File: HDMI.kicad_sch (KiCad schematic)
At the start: 8 parts, among them IC8 TPS2557QDRBTQ1, J4 HDMI_D_1.4

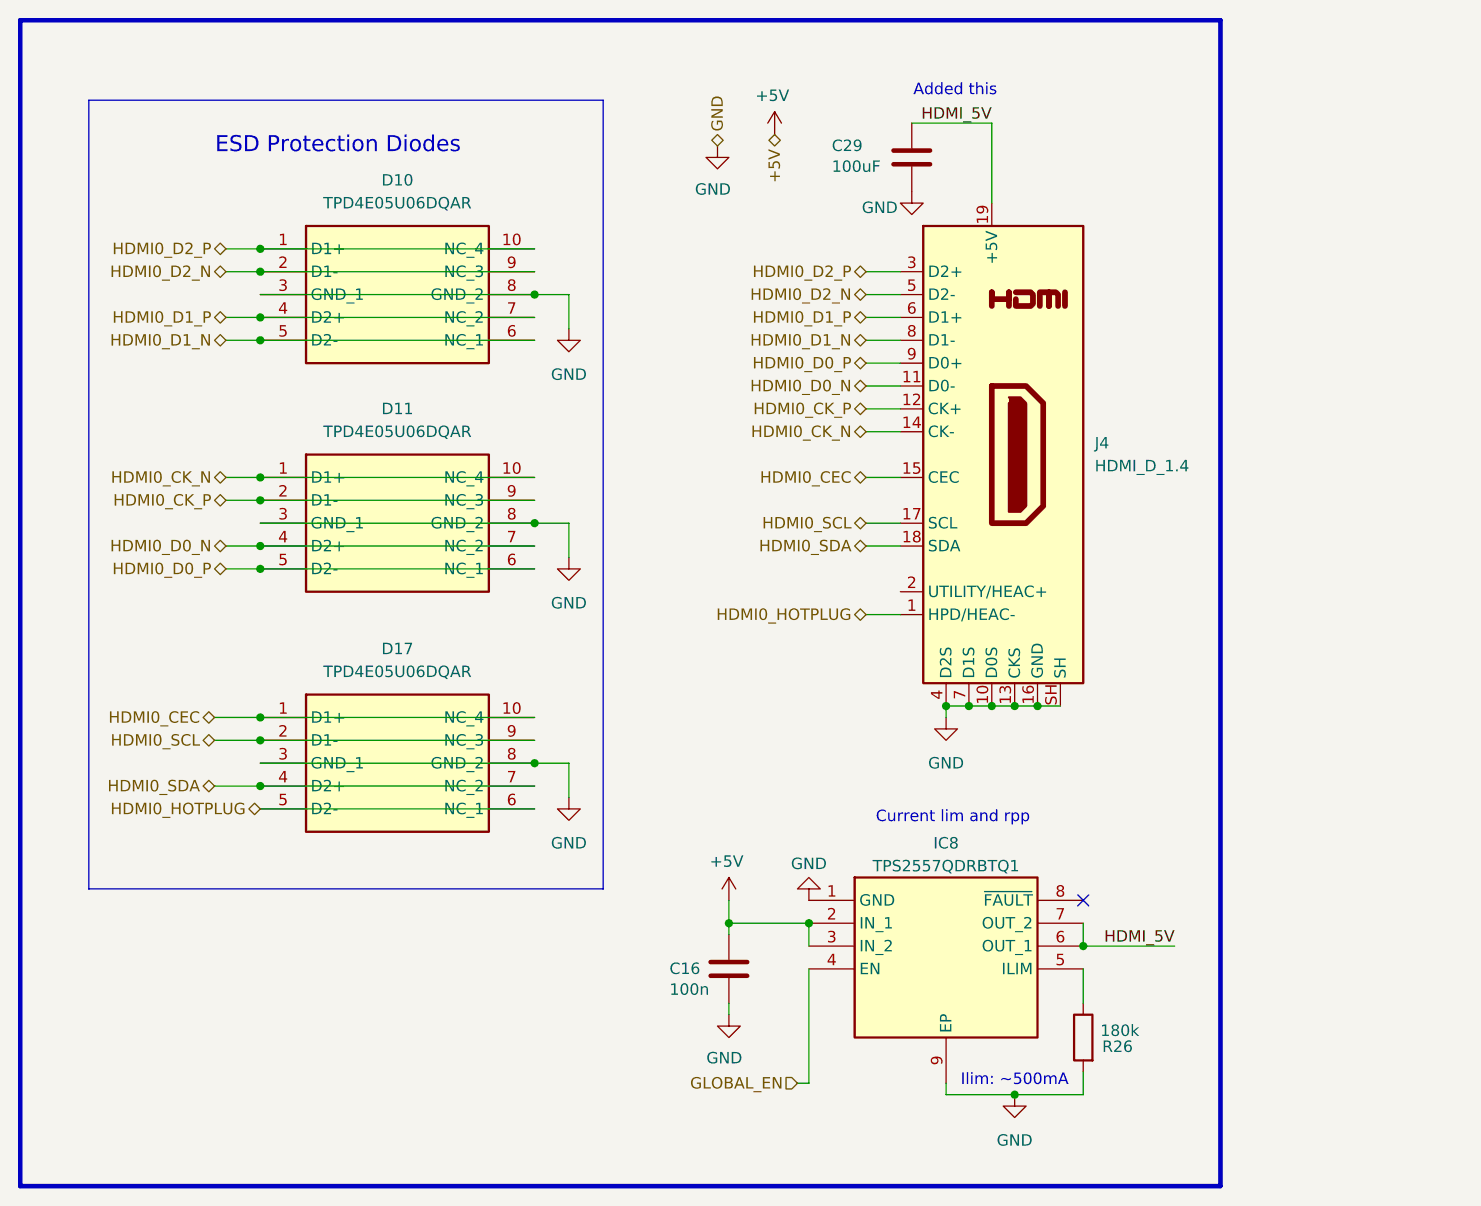
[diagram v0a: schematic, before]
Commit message: wow everything could not be worse
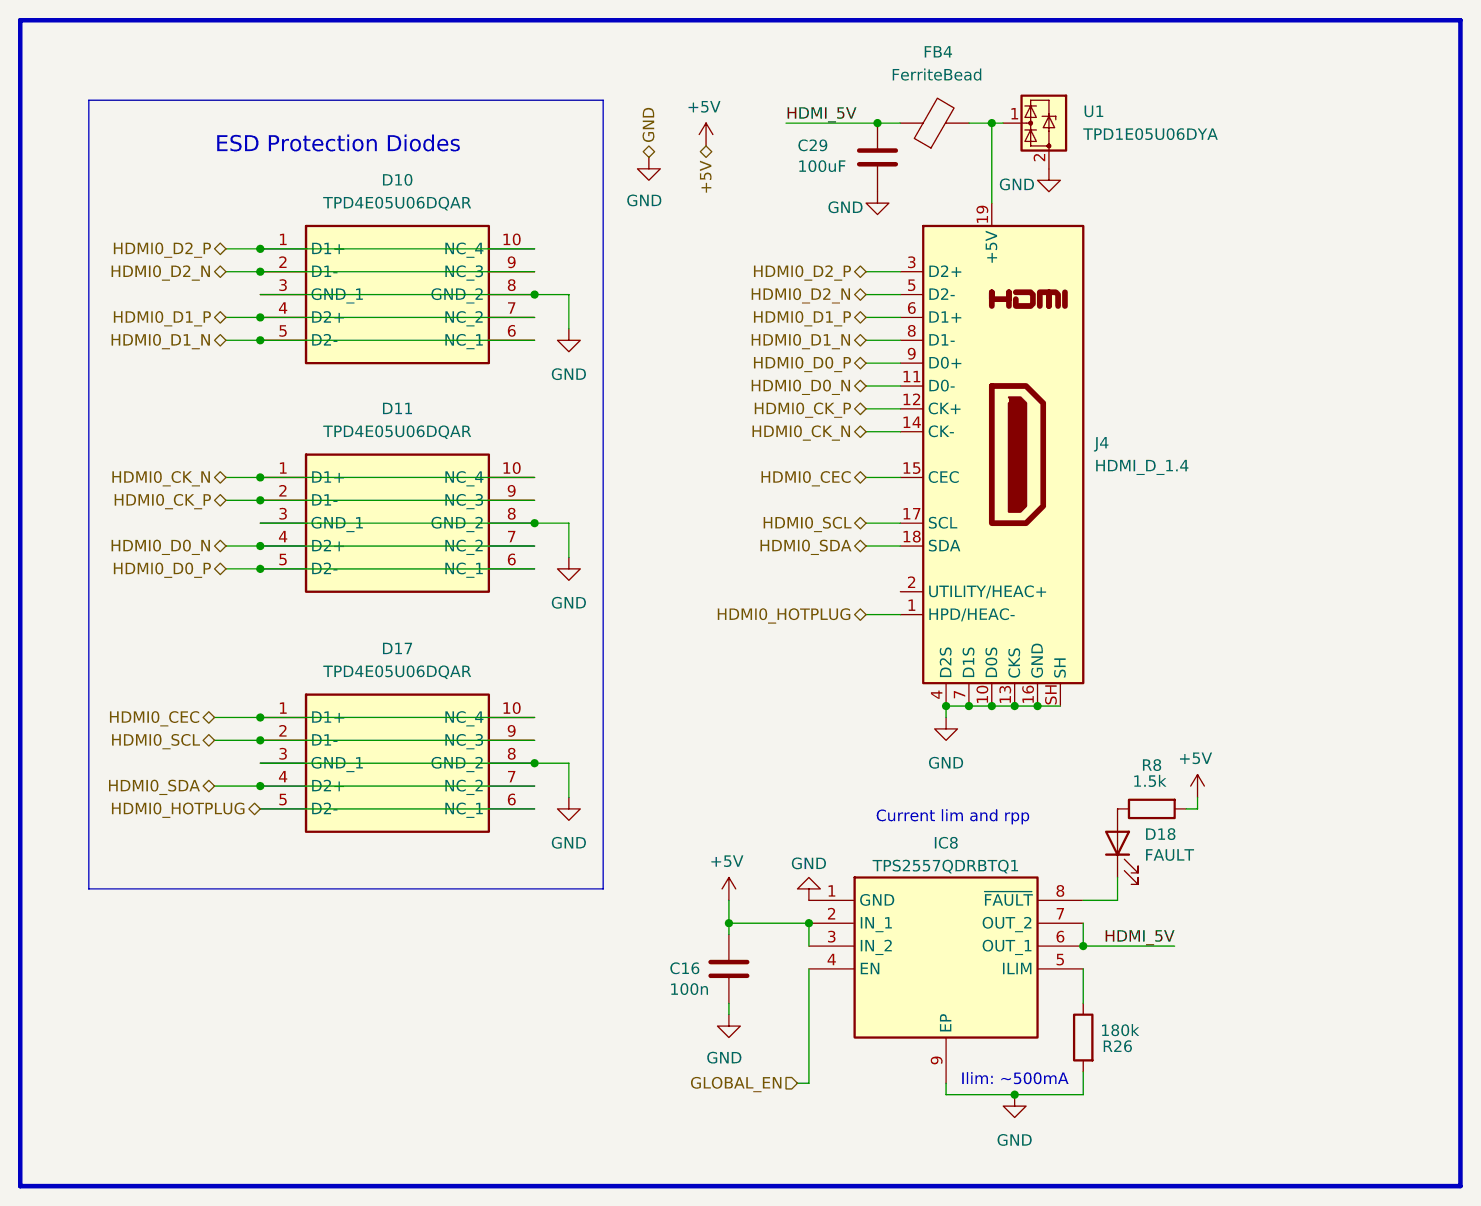
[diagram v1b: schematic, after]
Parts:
- added D18: FAULT, LED_SMD:LED_0603_1608Metric_Pad1.05x0.95mm_HandSolder, symbol Device:LED
- added FB4: FerriteBead, Inductor_SMD:L_1206_3216Metric, symbol Device:FerriteBead
- added R8: 1.5k, Resistor_SMD:R_0603_1608Metric_Pad0.98x0.95mm_HandSolder, symbol Device:R
- added U1: TPD1E05U06DYA, Diode_SMD:D_SOD-523, symbol Power_Protection:TPD1E05U06DYA
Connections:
- net +5V: now also R8.2
- net GND: now also U1.2 (GND)
- net HDMI_5V: now also FB4.1; no longer J4.19 (+5V)
- net at IC8.8 (~{FAULT}): now also D18.1 (K)
- new net: D18.2 (A), R8.1
- new net: FB4.2, J4.19 (+5V), U1.1 (I/O)
- no-connect marks 1 -> 0
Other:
- note removed: "Added this"
- moved on the sheet: C29

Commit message: my life could not be worse right now
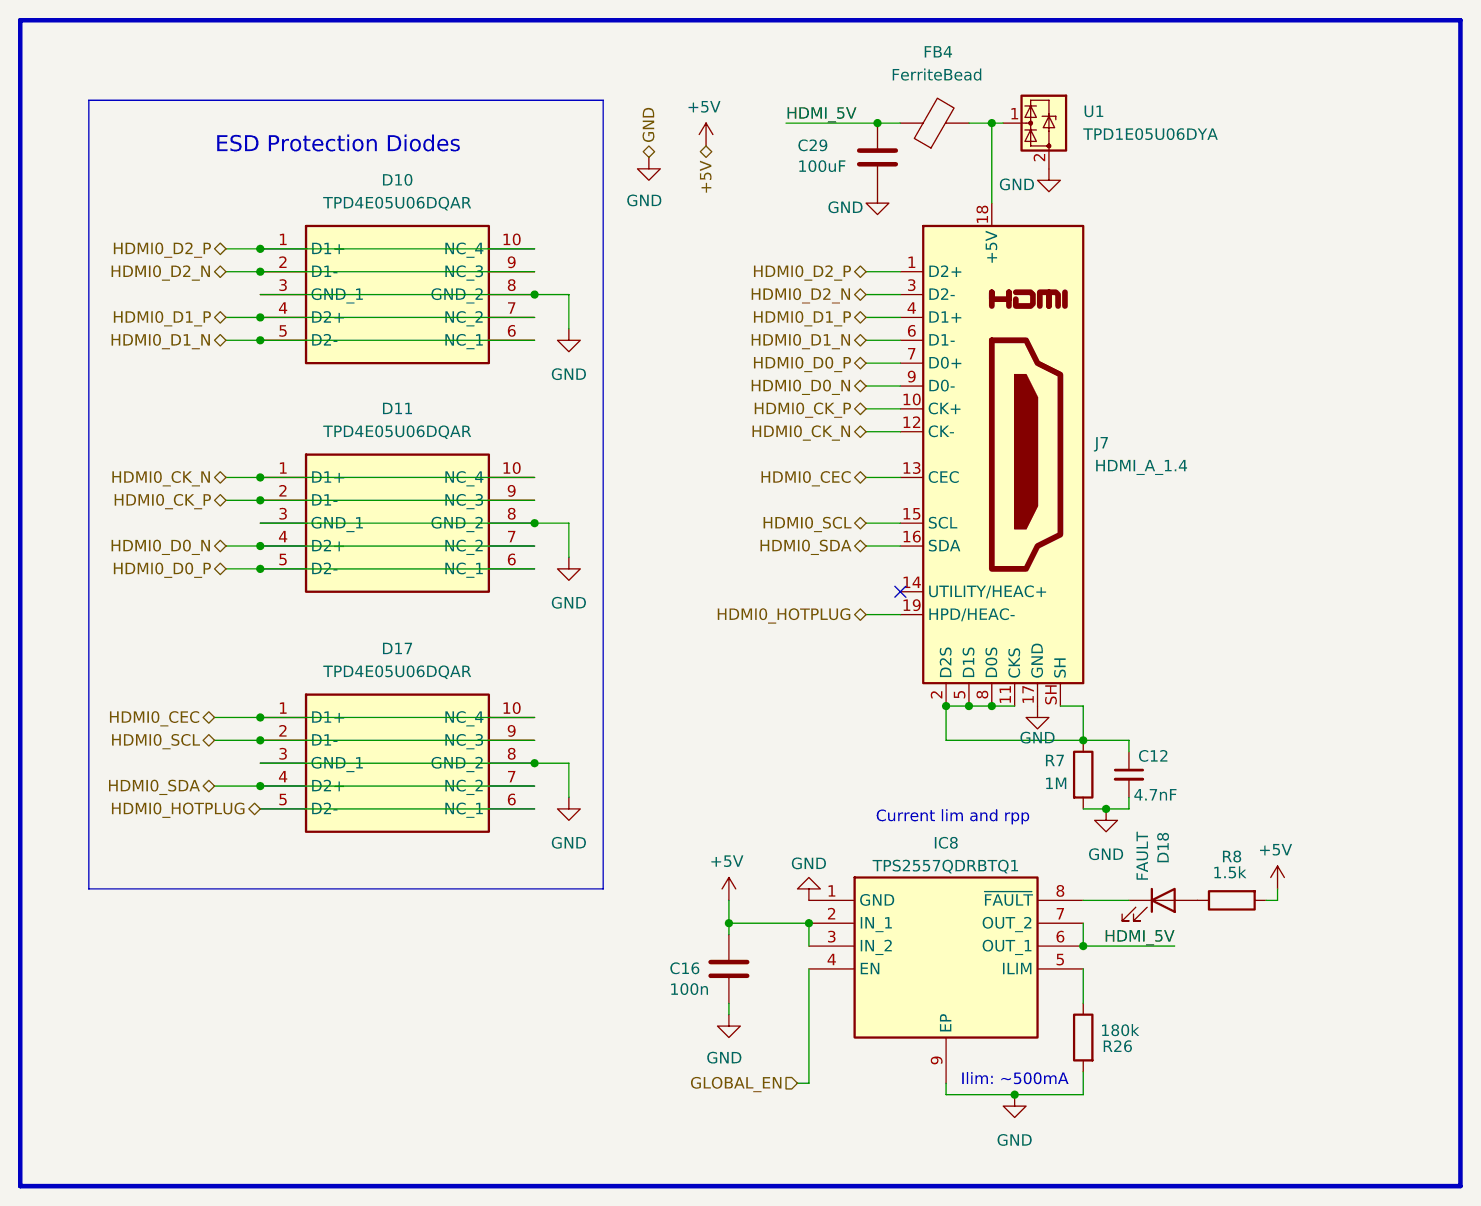
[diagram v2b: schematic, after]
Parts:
- removed J4: HDMI_D_1.4, Connector_Video:HDMI_Micro-D_Molex_46765-1x01, symbol Connector:HDMI_D_1.4
- added C12: 4.7nF, Capacitor_SMD:C_0603_1608Metric_Pad1.08x0.95mm_HandSolder, symbol Device:C_Small
- added J7: HDMI_A_1.4, Connector_Video:HDMI_A_Molex_208658-1001_Horizontal, symbol Connector:HDMI_A_1.4
- added R7: 1M, Resistor_SMD:R_0603_1608Metric_Pad0.98x0.95mm_HandSolder, symbol Device:R
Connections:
- net GND: now also C12.2, J7.17 (GND), R7.2
- net HDMI0_CEC: now also J7.13 (CEC)
- net HDMI0_CK_N: now also J7.12 (CK-)
- net HDMI0_CK_P: now also J7.10 (CK+)
- net HDMI0_D0_N: now also J7.9 (D0-)
- net HDMI0_D0_P: now also J7.7 (D0+)
- net HDMI0_D1_N: now also J7.6 (D1-)
- net HDMI0_D1_P: now also J7.4 (D1+)
- net HDMI0_D2_N: now also J7.3 (D2-)
- net HDMI0_D2_P: now also J7.1 (D2+)
- net HDMI0_HOTPLUG: now also J7.19 (HPD/HEAC-)
- net HDMI0_SCL: now also J7.15 (SCL)
- net HDMI0_SDA: now also J7.16 (SDA)
- net at FB4.2, U1.1 (I/O): now also J7.18 (+5V)
- new net: C12.1, J7.11 (CKS), J7.2 (D2S), J7.5 (D1S), J7.8 (D0S), J7.SH, R7.1
- no-connect marks 0 -> 1
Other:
- moved on the sheet: D18, R8

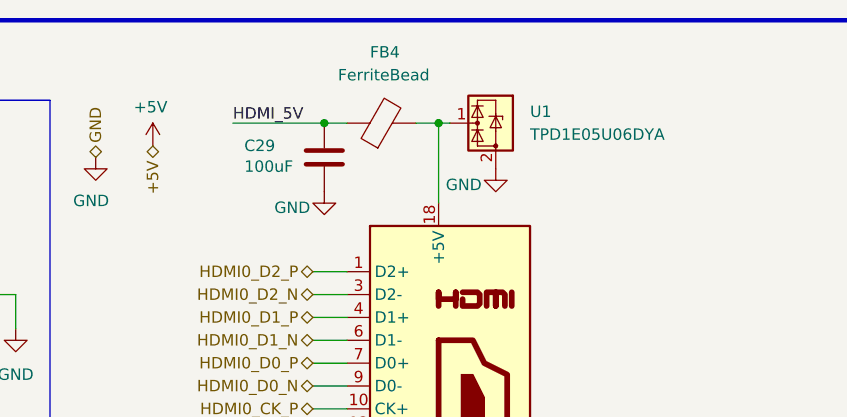
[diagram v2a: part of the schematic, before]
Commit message: frink2
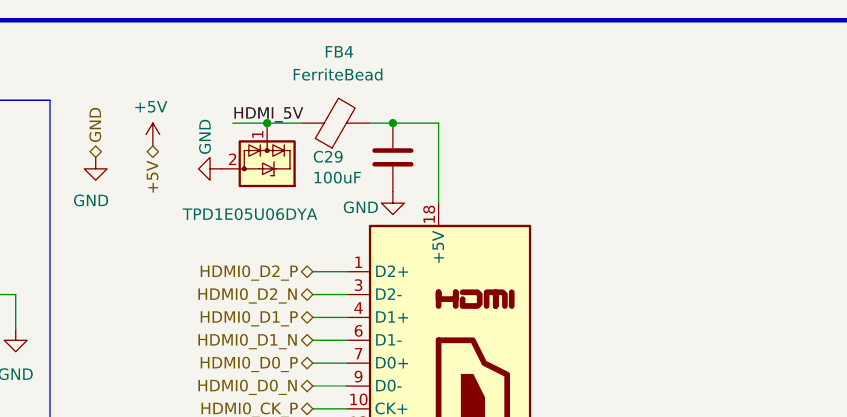
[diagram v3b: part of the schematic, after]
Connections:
- net HDMI_5V: now also U1.1 (I/O); no longer C29.1
- net at FB4.2, J7.18 (+5V): now also C29.1; no longer U1.1 (I/O)
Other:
- moved on the sheet: C29, FB4
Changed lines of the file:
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@@
-	)
-	(junction
-		(at 186.69 39.37)
-		(diameter 0)
-		(color 0 0 0 0)
 	)
 	(junction
@@
 	)
 	(junction
+		(at 181.61 39.37)
+		(diameter 0)
+		(color 0 0 0 0)
+	)
+	(junction
+		(at 167.64 39.37)
+		(diameter 0)
+		(color 0 0 0 0)
+	)
+	(junction
 		(at 189.23 147.32)
 		(diameter 0)
@@
 		(color 0 0 0 0)
 	)
-	(junction
-		(at 173.99 39.37)
-		(diameter 0)
-		(color 0 0 0 0)
-	)
 	(no_connect
 		(at 176.53 91.44)
@@
 	(wire
 		(pts
+			(xy 167.64 39.37) (xy 171.45 39.37)
+		)
+		(stroke
+			(width 0)
+			(type default)
+		)
+	)
+	(wire
+		(pts
 			(xy 105.41 60.96) (xy 135.89 60.96)
 		)
@@
 	(wire
 		(pts
-			(xy 187.96 39.37) (xy 186.69 39.37)
-		)
-		(stroke
-			(width 0)
-			(type default)
-		)
-	)
-	(wire
-		(pts
 			(xy 189.23 147.32) (xy 196.85 147.32)
 		)
@@
 	(wire
 		(pts
-			(xy 173.99 39.37) (xy 176.53 39.37)
-		)
-		(stroke
-			(width 0)
-			(type default)
-		)
-	)
-	(wire
-		(pts
 			(xy 172.72 93.98) (xy 176.53 93.98)
 		)
@@
 	(wire
 		(pts
+			(xy 181.61 39.37) (xy 186.69 39.37)
+		)
+		(stroke
+			(width 0)
+			(type default)
+		)
+	)
+	(wire
+		(pts
+			(xy 179.07 39.37) (xy 181.61 39.37)
+		)
+		(stroke
+			(width 0)
+			(type default)
+		)
+	)
+	(wire
+		(pts
 			(xy 181.61 104.14) (xy 184.15 104.14)
 		)
@@
 	(wire
 		(pts
-			(xy 184.15 39.37) (xy 186.69 39.37)
-		)
-		(stroke
-			(width 0)
-			(type default)
-		)
-	)
-	(wire
-		(pts
 			(xy 207.01 130.81) (xy 196.85 130.81)
 		)
@@
 	(wire
 		(pts
-			(xy 163.83 39.37) (xy 173.99 39.37)
+			(xy 163.83 39.37) (xy 167.64 39.37)
 		)
 		(stroke
@@
 	(symbol
 		(lib_id "power:GND")
-		(at 173.99 46.99 0)
+		(at 181.61 46.99 0)
 		(unit 1)
 		(exclude_from_sim no)
@@
 		(dnp no)
 		(property "Reference" "#PWR041"
-			(at 173.99 53.34 0)
+			(at 181.61 53.34 0)
 			(effects
 				(font
@@
 		)
 		(property "Value" "GND"
-			(at 170.434 48.768 0)
+			(at 178.054 48.768 0)
 			(effects
 				(font
@@
 		)
 		(property "Footprint" ""
-			(at 173.99 46.99 0)
+			(at 181.61 46.99 0)
 			(effects
 				(font
@@
 		)
 		(property "Datasheet" ""
-			(at 173.99 46.99 0)
+			(at 181.61 46.99 0)
 			(effects
 				(font
@@
 		)
 		(property "Description" "Power symbol creates a global label with name \"GND\" , ground"
-			(at 173.99 46.99 0)
+			(at 181.61 46.99 0)
 			(effects
 				(font
@@
 	(symbol
 		(lib_id "Device:C")
-		(at 173.99 43.18 0)
+		(at 181.61 43.18 0)
 		(unit 1)
 		(exclude_from_sim no)
@@
 		(dnp no)
 		(property "Reference" "C29"
-			(at 165.1 41.8846 0)
+			(at 172.72 43.1546 0)
 			(effects
 				(font
@@
 		)
 		(property "Value" "100uF"
-			(at 165.1 44.196 0)
+			(at 172.72 45.466 0)
 			(effects
 				(font
@@
 		)
 		(property "Footprint" "Capacitor_SMD:C_0805_2012Metric_Pad1.18x1.45mm_HandSolder"
-			(at 174.9552 46.99 0)
+			(at 182.5752 46.99 0)
 			(effects
 				(font
@@
 		)
 		(property "Datasheet" "https://content.kemet.com/datasheets/KEM_C1002_X7R_SMD.pdf"
-			(at 173.99 43.18 0)
+			(at 181.61 43.18 0)
 			(effects
 				(font
@@
 		)
 		(property "Description" "Unpolarized capacitor"
-			(at 173.99 43.18 0)
+			(at 181.61 43.18 0)
 			(effects
 				(font
@@
 		)
 		(property "P/N" "C0805C104M5RACTU"
-			(at 173.99 43.18 0)
+			(at 181.61 43.18 0)
 			(effects
 				(font
@@
 	(symbol
 		(lib_id "Device:FerriteBead")
-		(at 180.34 39.37 90)
+		(at 175.26 39.37 90)
 		(unit 1)
 		(exclude_from_sim no)
@@
 		(dnp no)
 		(property "Reference" "FB4"
-			(at 182.372 31.496 90)
+			(at 177.292 31.496 90)
 			(effects
 				(font
@@
 		)
 		(property "Value" "FerriteBead"
-			(at 180.594 34.036 90)
+			(at 175.514 34.036 90)
 			(effects
 				(font
@@
 		)
 		(property "Footprint" "Inductor_SMD:L_1206_3216Metric"
-			(at 180.34 41.148 90)
+			(at 175.26 41.148 90)
 			(effects
 				(font
@@
 		)
 		(property "Datasheet" "https://www.te.com/commerce/DocumentDelivery/DDEController?Action=srchrtrv&DocNm=1773178-3&DocType=Data%20Sheet&DocLang=English&DocFormat=pdf&PartCntxt=2-2176745-0"
-			(at 180.34 39.37 0)
+			(at 175.26 39.37 0)
 			(effects
 				(font
@@
 		)
 		(property "Description" "Ferrite bead"
-			(at 180.34 39.37 0)
+			(at 175.26 39.37 0)
 			(effects
 				(font
@@
 		)
 		(property "P/N" "BMC-Q2CY0220H "
-			(at 180.34 39.37 0)
+			(at 175.26 39.37 0)
 			(effects
 				(font
@@
 	(symbol
 		(lib_id "Power_Protection:TPD1E05U06DYA")
-		(at 193.04 39.37 270)
+		(at 167.64 44.45 180)
 		(unit 1)
 		(exclude_from_sim no)
@@
 		(on_board yes)
 		(dnp no)
-		(fields_autoplaced yes)
 		(property "Reference" "U1"
-			(at 196.85 38.0999 90)
+			(at 168.9101 48.26 90)
 			(effects
 				(font
@@
 				)
 				(justify left)
+				(hide yes)
 			)
 		)
 		(property "Value" "TPD1E05U06DYA"
-			(at 196.85 40.6399 90)
+			(at 173.228 49.53 0)
 			(effects
 				(font
@@
 		)
 		(property "Footprint" "Diode_SMD:D_SOD-523"
-			(at 188.595 41.91 0)
+			(at 165.1 40.005 0)
 			(effects
 				(font
@@
 		)
 		(property "Datasheet" "https://www.ti.com/lit/ds/symlink/tpd1e05u06.pdf"
-			(at 186.69 41.91 0)
+			(at 165.1 38.1 0)
 			(effects
 				(font
@@
 		)
 		(property "Description" "1-Channel ESD Protection for Super-Speed USB 3.0 Interface, SOD-523"
-			(at 193.04 39.37 0)
+			(at 167.64 44.45 0)
 			(effects
 				(font
@@
 		)
 		(instances
-			(project ""
+			(project "PiBoard"
 				(path "/e4d65698-b8ec-4bf6-9f2b-a5010377155a/2dec5fd6-8756-425d-9ae9-2f1c2fc4e6c1/3504b936-9c0d-4baf-9c43-98590fac5230"
 					(reference "U1")
@@
 	(symbol
 		(lib_id "power:GND")
-		(at 193.04 44.45 0)
+		(at 162.56 44.45 270)
 		(unit 1)
 		(exclude_from_sim no)
@@
 		(dnp no)
 		(property "Reference" "#PWR042"
-			(at 193.04 50.8 0)
+			(at 156.21 44.45 0)
 			(effects
 				(font
@@
 		)
 		(property "Value" "GND"
-			(at 189.484 46.228 0)
+			(at 160.782 40.894 0)
 			(effects
 				(font
@@
 		)
 		(property "Footprint" ""
-			(at 193.04 44.45 0)
+			(at 162.56 44.45 0)
 			(effects
 				(font
@@
 		)
 		(property "Datasheet" ""
-			(at 193.04 44.45 0)
+			(at 162.56 44.45 0)
 			(effects
 				(font
@@
 		)
 		(property "Description" "Power symbol creates a global label with name \"GND\" , ground"
-			(at 193.04 44.45 0)
-			(effects
-				(font
+			(at 162.56 44.45 0)
+			(effects
+				(font
